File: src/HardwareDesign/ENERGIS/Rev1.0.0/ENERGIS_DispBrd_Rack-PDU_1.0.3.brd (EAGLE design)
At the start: 124 x 40 mm, 65 parts, among them CON1 FPC40-HD, CON2 AFC11-S20ICC-00, IC1 MCP23017-E/ML, IC2 MCP23017-E/ML, T1 BSS138

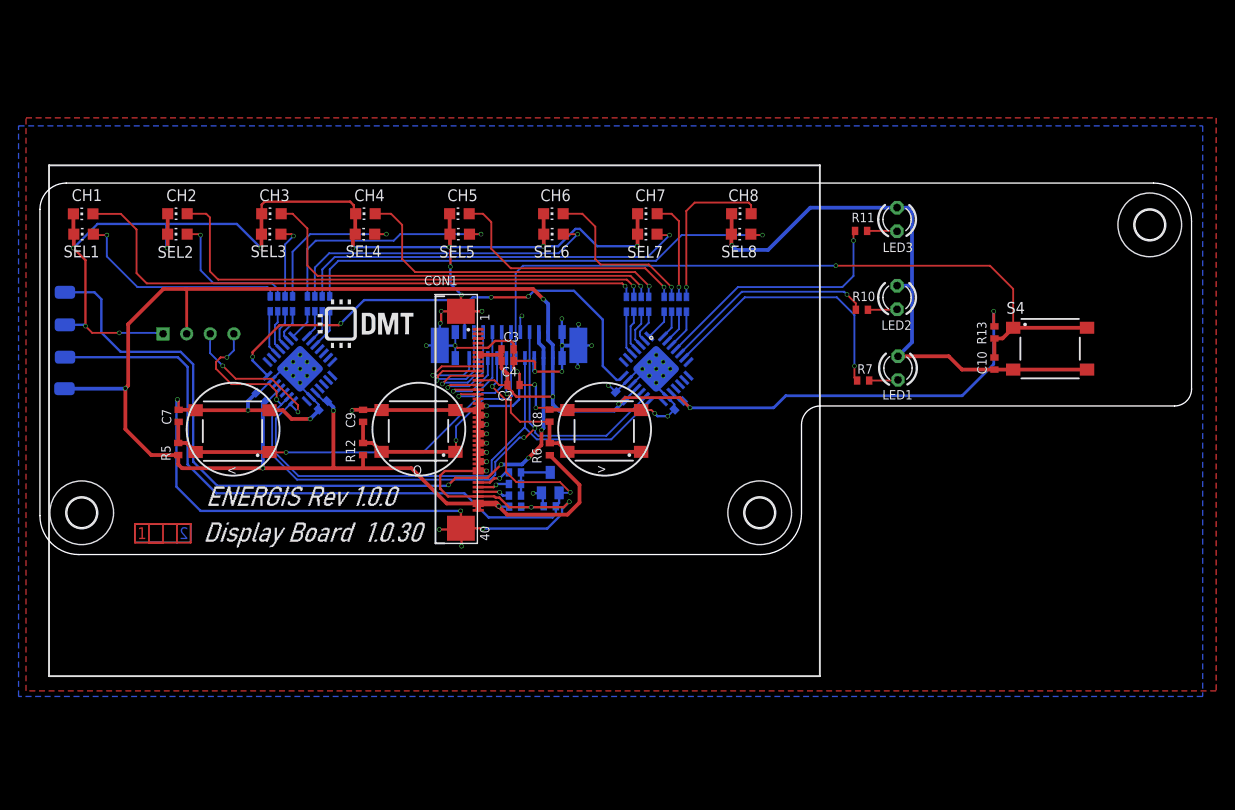
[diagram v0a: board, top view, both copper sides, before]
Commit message: update software, bugfix
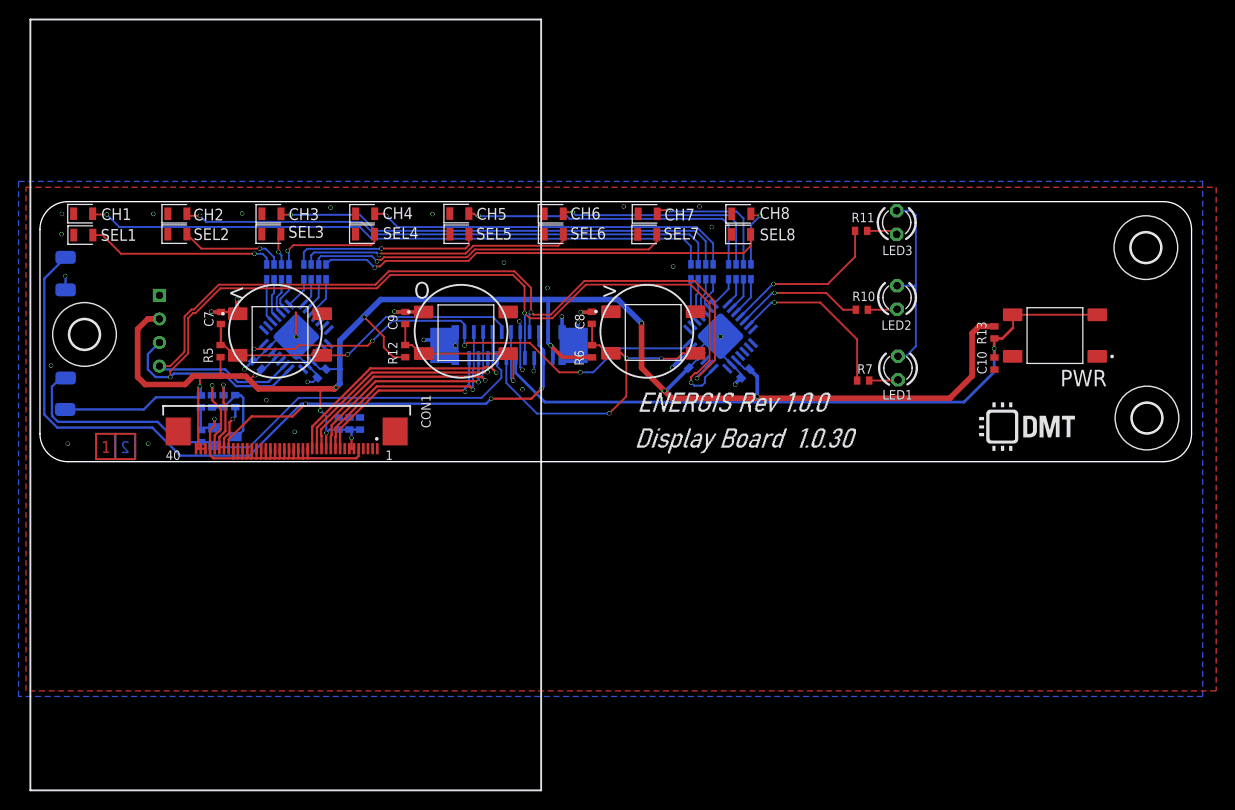
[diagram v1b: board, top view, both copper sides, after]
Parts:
- removed S4: TC-6601-5.0-160, Wurth_Switch_WS-TASV:430182043816
- added PWR: TS-1002S-04326C, ds_passive:PUSHBUTTON-6X6
- <, >, O: value TC-6601-5.0-160 -> TS-1002S-04326C; device Wurth_Switch_WS-TASV:430182043816 -> ds_passive:PUSHBUTTON-6X6
- C1, C3: value 10uF -> DNI
- C10, C11, C12, C5, C6, C7, C8, C9: value 100nF -> 100nF 50V; device ds_passive:C0402 -> ds_capacitors:0402
- C2, C4: value 100nF -> DNI
- CH1, CH2, CH3, CH4, CH5, CH6, CH7, CH8: value (none) -> Green; device led:CHIP-LED0805 -> ds_LED:LED-0805
- CON1: value FPC40-HD -> DNI
- CON2: value AFC11-S20ICC-00 -> AFC11-S20ICC-00
- DSP: value (none) -> DNI
- IC1, IC2: value MCP23017-E/ML -> MCP23017T-E/ML
- LED1: value (none) -> GREEN; device led:LED3MM -> ds_LED:LED3MM
- LED2: value XL-2012UBC -> BLUE; device led:LED3MM -> ds_LED:LED3MM
- LED3: value XL-2012SURC -> RED; device led:LED3MM -> ds_LED:LED3MM
- R1, R2, R3: value 56R -> DNI
- R10, R11, R7: value 1K -> 1K 1%; device ds_passive:0402 -> ds_resistor:0402
- R12, R13, R4, R5, R6: value 10K -> 10K 1%; device ds_passive:0402 -> ds_resistor:0402
- R14, R15, R8, R9: value 4D03WGJ0102T5E 1K -> 1K 1%; device Resistor Array:742C083103JP -> ds_resistor:_0603X4-1206
- SEL1, SEL2, SEL3, SEL4, SEL5, SEL6, SEL7, SEL8: value (none) -> Orange; device led:CHIP-LED0805 -> ds_LED:LED-0805
- moved U$5 72.1 mm to (107.6, 27.7)
- moved U$2 42.9 mm to (123.2, 28.7)
- moved R4 38.3 mm to (21.4, 26.8), turned to 90 degrees
- moved C1 35.7 mm to (21.3, 30.5), turned to 270 degrees
- moved T1 35.4 mm to (23.9, 26.7), turned to 90 degrees
- moved R3 34.2 mm to (22.5, 30.5), turned to 90 degrees
- moved R2 32.6 mm to (23.8, 30.5), turned to 90 degrees
- moved R1 31.1 mm to (25.0, 30.5), turned to 270 degrees
- moved CON1 21.8 mm to (30.1, 49.6), turned to 270 degrees
- moved C3 19.8 mm to (36.2, 28.1), flipped to the bottom, turned to 90 degrees
- moved U$4 19.2 mm to (8.80, 37.7)
- moved C4 18.3 mm to (37.3, 28.1), flipped to the bottom, turned to 90 degrees
- moved C2 17.0 mm to (38.5, 28.1), flipped to the bottom, turned to 90 degrees
- moved > 11.8 mm to (70.0, 37.9), turned to 0 degrees
- moved O 11.7 mm to (49.9, 37.9), turned to 0 degrees
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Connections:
- net GND: now also <.1, >.1, O.1, PWR.1, PWR.2; no longer <.4, >.4, O.4, S4.2, S4.4
- net KEY_0: now also <.4; no longer <.1
- net KEY_1: now also >.4; no longer >.1
- net KEY_2: now also O.4; no longer O.1
- net KEY_3: now also PWR.3, PWR.4; no longer S4.1, S4.3
- net N$10: now also R14.B1; no longer R14.2
- net N$11: now also R14.A1; no longer R14.1
- net N$12: now also R15.D1; no longer R15.4
- net N$13: now also R15.C1; no longer R15.3
- net N$14: now also R15.B1; no longer R15.2
- net N$15: now also R15.A1; no longer R15.1
- net N$16: now also R14.D2; no longer R14.5
- net N$17: now also R14.C2; no longer R14.6
- net N$18: now also R14.B2; no longer R14.7
- net N$19: now also R14.A2; no longer R14.8
- net N$20: now also R15.D2; no longer R15.5
- net N$21: now also R15.C2; no longer R15.6
- net N$22: now also R15.B2; no longer R15.7
- net N$23: now also R15.A2; no longer R15.8
- net N$50: now also R8.D1; no longer R8.4
- net N$51: now also R8.C1; no longer R8.3
- net N$52: now also R8.B1; no longer R8.2
- net N$53: now also R8.A1; no longer R8.1
- net N$54: now also R9.D1; no longer R9.4
- net N$55: now also R9.C1; no longer R9.3
- net N$56: now also R9.B1; no longer R9.2
- net N$57: now also R9.A1; no longer R9.1
- net N$58: now also R8.D2; no longer R8.5
- net N$59: now also R8.C2; no longer R8.6
- net N$60: now also R8.B2; no longer R8.7
- net N$61: now also R8.A2; no longer R8.8
- net N$62: now also R9.D2; no longer R9.5
- net N$63: now also R9.C2; no longer R9.6
- net N$64: now also R9.B2; no longer R9.7
- net N$65: now also R9.A2; no longer R9.8
- net N$8: now also R14.D1; no longer R14.4
- net N$9: now also R14.C1; no longer R14.3
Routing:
- net GND: track 429.7 -> 123.6 mm, vias 68 -> 37
- net +3V3: track 245.4 -> 199.2 mm, vias 9 -> 11
- net I2C0_SCL: track 76.2 -> 109.6 mm, vias 2 -> 3
- net LCD_BL: track 90.9 -> 60.2 mm, vias 2 -> 0
- net I2C0_SDA: track 78.4 -> 100.5 mm, vias 4 -> 2
- net LCD_RES: track 11.6 -> 29.7 mm
- net LCD_MISO: track 9.03 -> 24.7 mm
- net LCD_MOSI: track 12.2 -> 27.7 mm
- net KEY_1: track 23.2 -> 36.2 mm, vias 1 -> 3
- net LCD_SCLK: track 10.2 -> 23.0 mm
- net LCD_DC: track 13.7 -> 25.3 mm
- net +5V: track 82.5 -> 93.5 mm, vias 4 -> 3
- net N$65: track 17.7 -> 6.81 mm
- net KEY_0: track 46.3 -> 35.8 mm
- net LCD_CS: track 10.7 -> 21.1 mm
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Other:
- board size 124 x 40 mm -> 124 x 28 mm
- board text removed: "4"

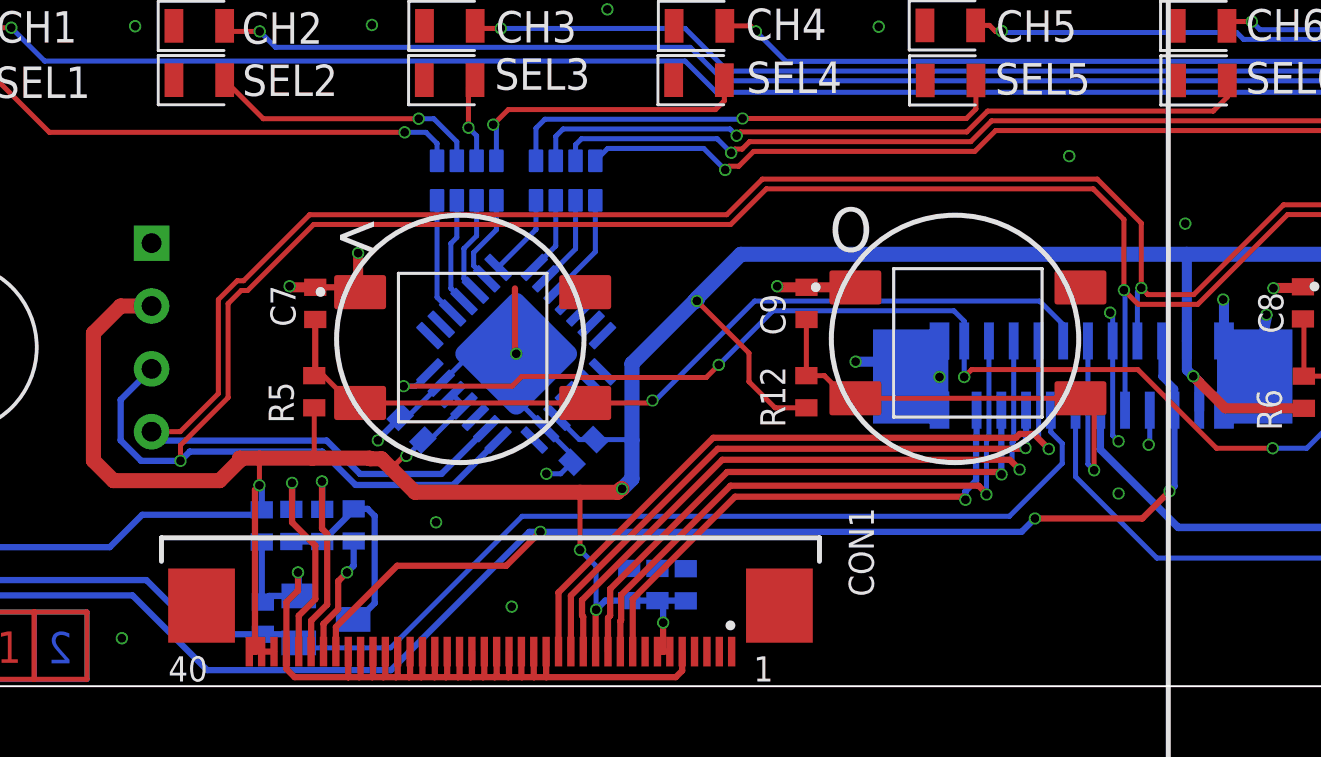
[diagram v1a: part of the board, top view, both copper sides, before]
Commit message: Baseline commit. Device is functioning as expected, software is working
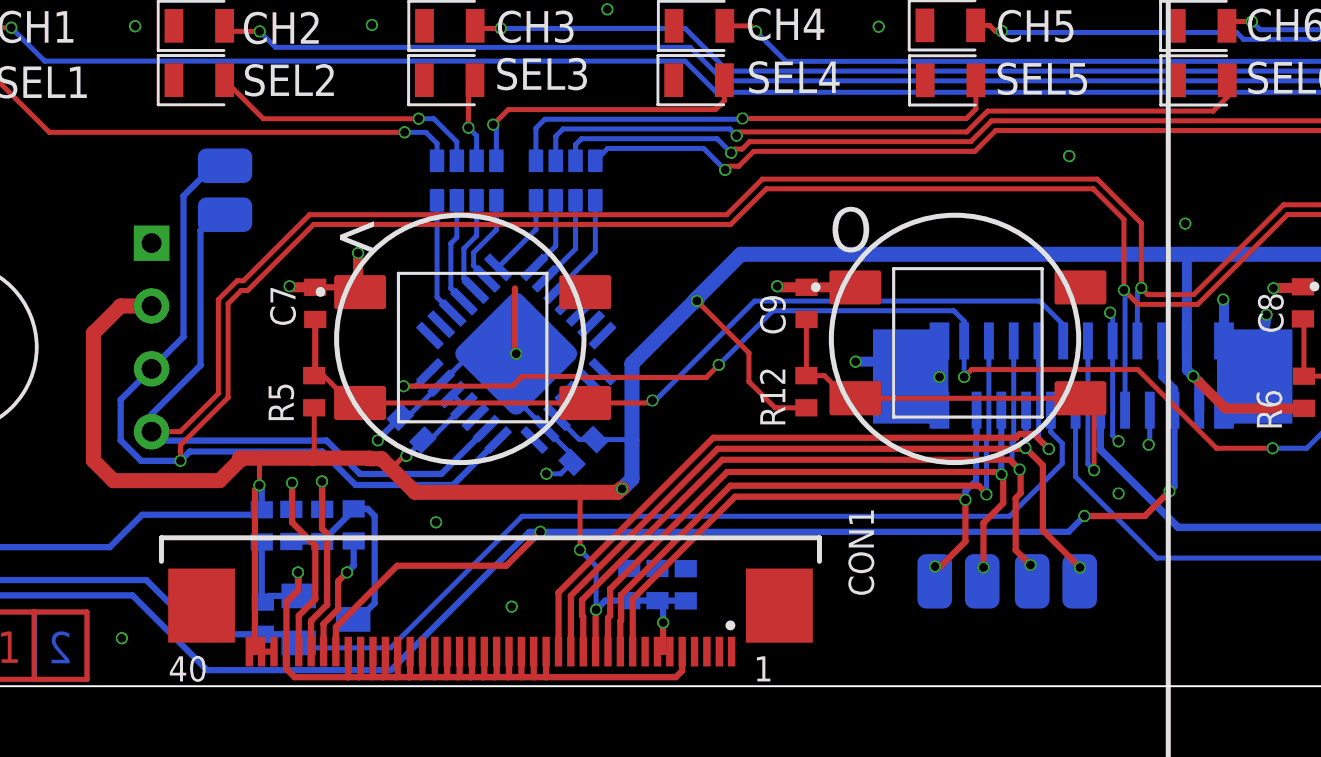
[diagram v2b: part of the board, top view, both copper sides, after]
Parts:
- added CS, MISO, MOSI, SCK, SCL0, SDA0: TP, ds_passive:TP
- renumbered TP1 to 3V3, TP16 to GND, TP2 to 5V, TP3 to BL
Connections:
- net I2C0_SCL: now also SCL0.TP
- net I2C0_SDA: now also SDA0.TP
- net LCD_CS: now also CS.TP
- net LCD_MISO: now also MISO.TP
- net LCD_MOSI: now also MOSI.TP
- net LCD_SCLK: now also SCK.TP
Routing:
- net I2C0_SDA: track 100.5 -> 110.7 mm
- net I2C0_SCL: track 109.6 -> 119.3 mm
- net LCD_MISO: track 24.7 -> 31.0 mm, vias 1 -> 2
- net LCD_MOSI: track 27.7 -> 32.6 mm, vias 1 -> 2
- net LCD_SCLK: track 23.0 -> 27.7 mm, vias 1 -> 2
- net LCD_CS: track 21.1 -> 25.1 mm, vias 1 -> 2
